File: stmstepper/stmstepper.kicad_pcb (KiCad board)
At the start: 2 copper layers, 50 x 50 mm, 4 parts, among them J1 Conn_02x12, J2 Conn_02x12, J3 Conn_02x12, J4 Conn_02x12

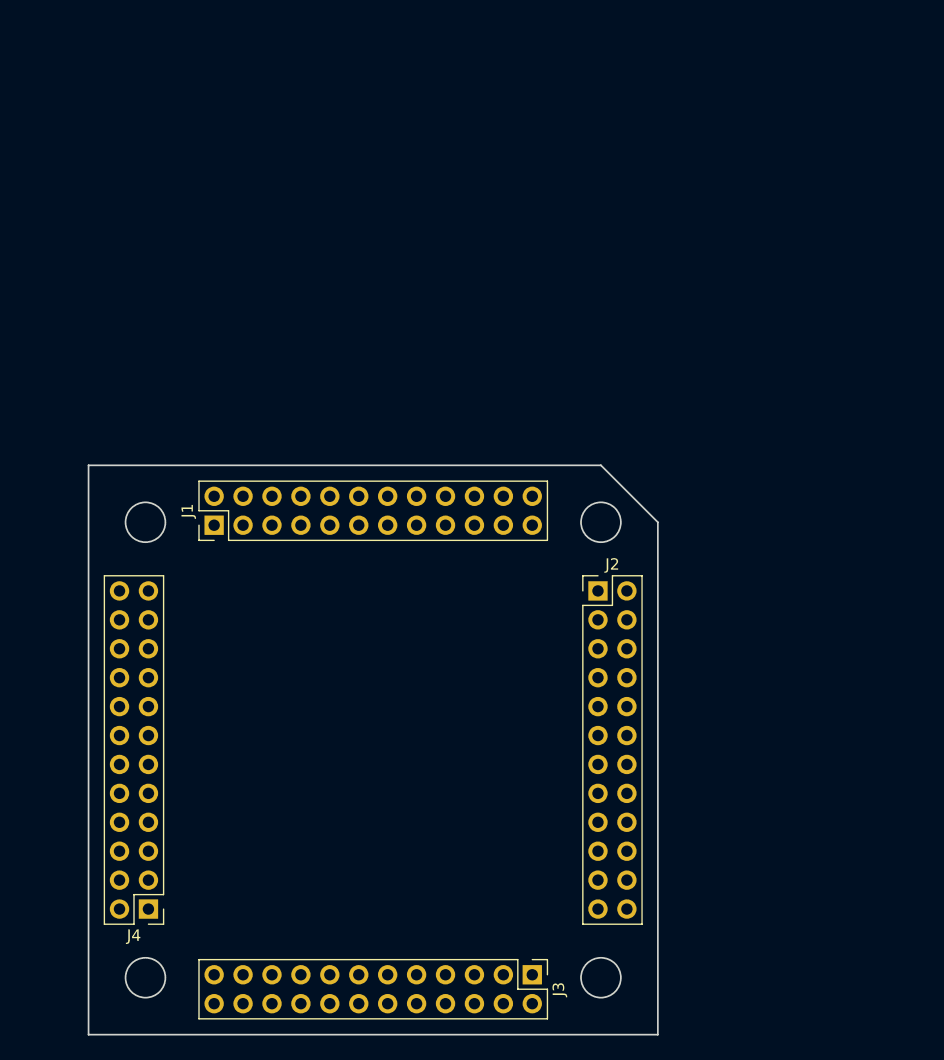
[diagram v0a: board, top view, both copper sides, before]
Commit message: add stmstepper pcb
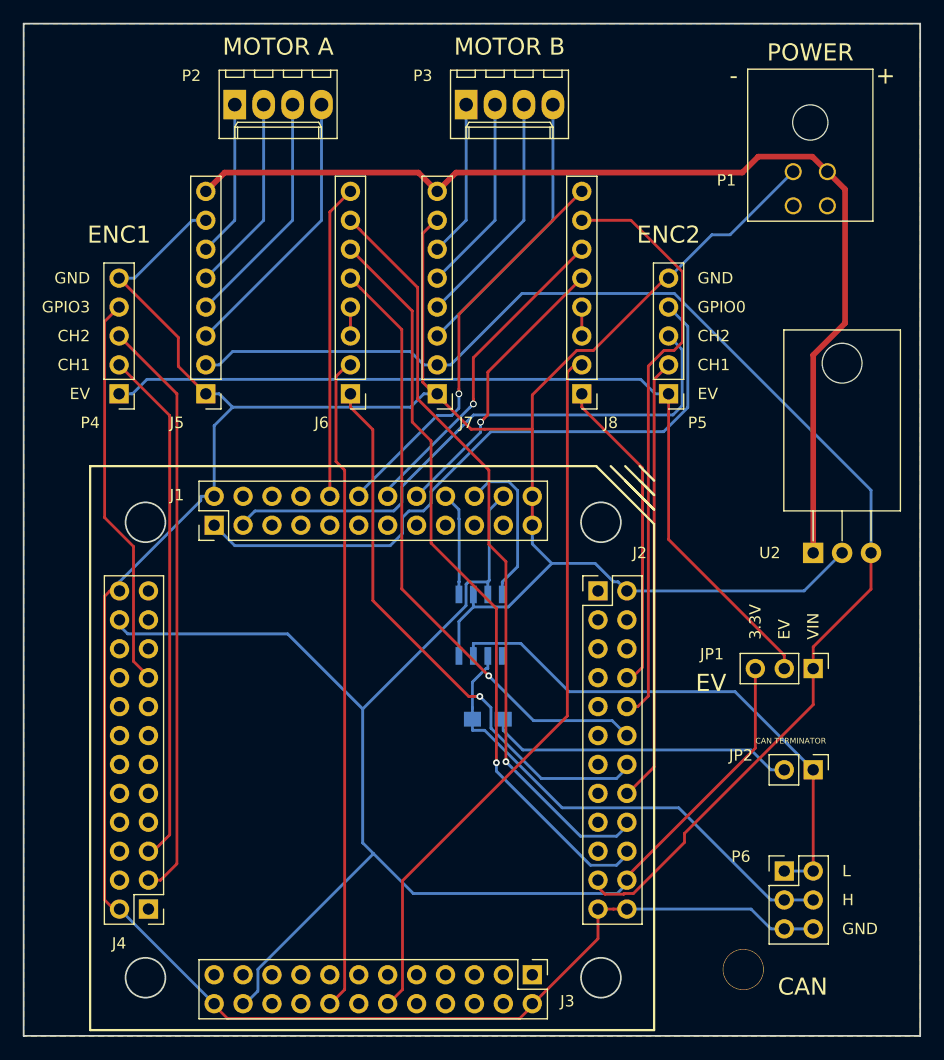
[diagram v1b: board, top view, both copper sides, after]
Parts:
- added J5: CONN_01X08, Socket_Strips:Socket_Strip_Straight_1x08_Pitch2.54mm, F.Cu at (130.3, 66.7)
- added J6: CONN_01X08, Socket_Strips:Socket_Strip_Straight_1x08_Pitch2.54mm, F.Cu at (143.0, 66.7)
- added J7: CONN_01X08, Socket_Strips:Socket_Strip_Straight_1x08_Pitch2.54mm, F.Cu at (150.6, 66.7)
- added J8: CONN_01X08, Socket_Strips:Socket_Strip_Straight_1x08_Pitch2.54mm, F.Cu at (163.3, 66.7)
- added JP1: Jumper_NC_Dual, Pin_Headers:Pin_Header_Straight_1x03_Pitch2.54mm, F.Cu at (183.6, 90.8)
- added JP2: Jumper, Pin_Headers:Pin_Header_Straight_1x02_Pitch2.54mm, F.Cu at (183.6, 99.7)
- added P1: CONN_01X02, Connectors_Molex:Molex_Microfit3_Header_02x02_Angled_43045-040x, F.Cu at (181.9, 47.2)
- added P2: CONN_01X04, Connectors_Molex:Molex_KK-6410-04_04x2.54mm_Straight, F.Cu at (132.8, 41.3)
- added P3: CONN_01X04, Connectors_Molex:Molex_KK-6410-04_04x2.54mm_Straight, F.Cu at (153.2, 41.3)
- added P4: CONN_01X05, Pin_Headers:Pin_Header_Straight_1x05_Pitch2.54mm, F.Cu at (122.7, 66.7)
- added P5: CONN_01X05, Pin_Headers:Pin_Header_Straight_1x05_Pitch2.54mm, F.Cu at (170.9, 66.7)
- added P6: Conn_02x03_Odd_Even, libs:CAN_Header, F.Cu at (181.1, 108.6)
- added R1: R120, Resistors_SMD:R_0805_HandSoldering, B.Cu at (155.1, 95.3)
- added U1: SN65HVD230, Housings_SOIC:SOIC-8_3.9x4.9mm_Pitch1.27mm, B.Cu at (154.4, 87.0)
- added U2: 7805, TO_SOT_Packages_THT:TO-220_Horizontal, F.Cu at (183.6, 80.7)
- J1, J2, J3, J4: value Conn_02x12 -> Conn_02x12_Odd_Even
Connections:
- J1 pad 1: (no net) -> /GPIO0
- J1 pad 10: (no net) -> /A-EN
- J1 pad 11: (no net) -> /GPIO10
- J1 pad 12: (no net) -> /B-EN
- J1 pad 13: (no net) -> /GPIO13
- J1 pad 14: (no net) -> /B-MS2
- J1 pad 15: (no net) -> /SPI3_MOSI
- J1 pad 16: (no net) -> /B-MS3
- J1 pad 17: (no net) -> /SPI3_MISO
- J1 pad 18: (no net) -> /CAN3_TX
- J1 pad 19: (no net) -> /SPI3_SCK
- J1 pad 20: (no net) -> /CAN3_RX
- J1 pad 21: (no net) -> Net-(J1-Pad21)
- J1 pad 3: (no net) -> /TIM4_CH2
- J1 pad 4: (no net) -> /GPIO11
- J1 pad 5: (no net) -> /QSPI_NCS
- J1 pad 6: (no net) -> /I2C1_SCL
- J1 pad 7: (no net) -> /QSPI_IO2
- J1 pad 8: (no net) -> /I2C1_SDA
- J1 pad 9: (no net) -> /QSPI_IO1
- J2 pad 1: (no net) -> /GPIO15
- J2 pad 10: (no net) -> /B-MS1
- J2 pad 11: (no net) -> /GPIO7
- J2 pad 12: (no net) -> /A-MS3
- J2 pad 13: (no net) -> /CAN1_TX
- J2 pad 14: (no net) -> /A-DIR
- J2 pad 15: (no net) -> /CAN1_RX
- J2 pad 16: (no net) -> /TIM4_CH1
- J2 pad 17: (no net) -> /UART5_TX
- J2 pad 18: (no net) -> /A-MS1
- J2 pad 19: (no net) -> /UART5_RX
- J2 pad 20: (no net) -> /A-MS2
- J2 pad 21: (no net) -> /VDD
- J2 pad 3: (no net) -> /TIM8_CH4
- J2 pad 4: (no net) -> /SWCLK
- J2 pad 5: (no net) -> /TIM8_CH3
- J2 pad 6: (no net) -> /SWDIO
- J2 pad 7: (no net) -> /TIM8_CH2
- J2 pad 8: (no net) -> /B-DIR
- J2 pad 9: (no net) -> /TIM8_CH1
- J3 pad 1: (no net) -> /TIM12_CH2
- J3 pad 10: (no net) -> /TIM1_CH2N
- J3 pad 11: (no net) -> /GPIO6
- J3 pad 12: (no net) -> /B-STEP
- J3 pad 13: (no net) -> /GPIO5
- J3 pad 14: (no net) -> /TIM1_CH1N
- J3 pad 15: (no net) -> /QSPI_CLK
- J3 pad 16: (no net) -> /A-STEP
- J3 pad 17: (no net) -> /ADC_IN14
- J3 pad 18: (no net) -> /SPI1_MOSI
- J3 pad 19: (no net) -> /SPI1_SCK
- J3 pad 20: (no net) -> /SPI1_MISO
- J3 pad 21: (no net) -> Net-(J3-Pad21)
- J3 pad 23: (no net) -> /DAC1_OUT
- J3 pad 3: (no net) -> /TIM12_CH1
- J3 pad 4: (no net) -> /TIM1_BKIN
- J3 pad 5: (no net) -> /I2C2_SCL
- J3 pad 6: (no net) -> /TIM1_CH3N
- J3 pad 7: (no net) -> /I2C2_SDA
- J3 pad 8: (no net) -> /TIM1_CH3
- J3 pad 9: (no net) -> /ADC_IN7
- J4 pad 1: (no net) -> /TIM3_CH4
- J4 pad 10: (no net) -> /NRST
- J4 pad 11: (no net) -> /SPI2_MISO
- J4 pad 12: (no net) -> /ADC_IN3
- J4 pad 13: (no net) -> /SPI2_SCK
- J4 pad 14: (no net) -> /ADC_IN2
- J4 pad 15: (no net) -> /GPIO4
- J4 pad 16: (no net) -> /VBAT
- J4 pad 17: (no net) -> /GPIO3
- J4 pad 18: (no net) -> /TIM9_CH2
- J4 pad 19: (no net) -> /GPIO2
- J4 pad 20: (no net) -> /TIM9_CH1
- J4 pad 21: (no net) -> Net-(J4-Pad21)
- J4 pad 23: (no net) -> /GPIO1
- J4 pad 3: (no net) -> /TIM2_CH2
- J4 pad 4: (no net) -> /TIM3_CH3
- J4 pad 5: (no net) -> /TIM2_CH1
- J4 pad 6: (no net) -> /ADC_IN13
- J4 pad 7: (no net) -> /ADC_IN10
- J4 pad 8: (no net) -> /ADC_IN15
- J4 pad 9: (no net) -> /SPI2_MOSI
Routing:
- net GND: track 0.00 -> 281.5 mm
- net /+3V3: track 0.00 -> 129.6 mm
- net /VDD: track 0.00 -> 117.2 mm
- net /VMOT: track 0.00 -> 93.0 mm
- net /EV: track 0.00 -> 77.7 mm
- net /A-MS1: track 0.00 -> 67.2 mm, vias 0 -> 1
- net /A-MS2: track 0.00 -> 66.7 mm, vias 0 -> 1
- net /B-STEP: track 0.00 -> 63.6 mm
- net /GPIO0: track 0.00 -> 58.3 mm
- net /A-STEP: track 0.00 -> 57.7 mm
- net /A-MS3: track 0.00 -> 54.3 mm, vias 0 -> 1
- net /B-MS1: track 0.00 -> 52.0 mm
- net /TIM2_CH2: track 0.00 -> 51.6 mm
- net /TIM4_CH2: track 0.00 -> 50.5 mm
- net /A-DIR: track 0.00 -> 49.5 mm, vias 0 -> 1
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- added copper zone on B.Cu, net GND
- added copper zone on F.Cu, net GND
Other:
- board size 50 x 50 mm -> 78.7 x 88.9 mm
- board text added: "+"
- board text added: "-"
- board text added: "3.3V"
- board text added: "CAN"
- board text added: "CAN TERMINATOR"
- board text added: "CH1"
- board text added: "CH2"
- board text added: "ENC1"
- board text added: "ENC2"
- board text added: "EV"
- board text added: "GND"
- board text added: "GPIO0"
- board text added: "GPIO3"
- board text added: "H"
- board text added: "L"
- board text added: "MOTOR A"
- board text added: "MOTOR B"
- board text added: "POWER"
- board text added: "VIN"
